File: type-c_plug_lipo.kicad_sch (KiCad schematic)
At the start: 14 parts, among them J1 Conn_Battery, J2 USB_C_Plug_USB2.0, J4 Conn_Pwr, U1 MCP73831

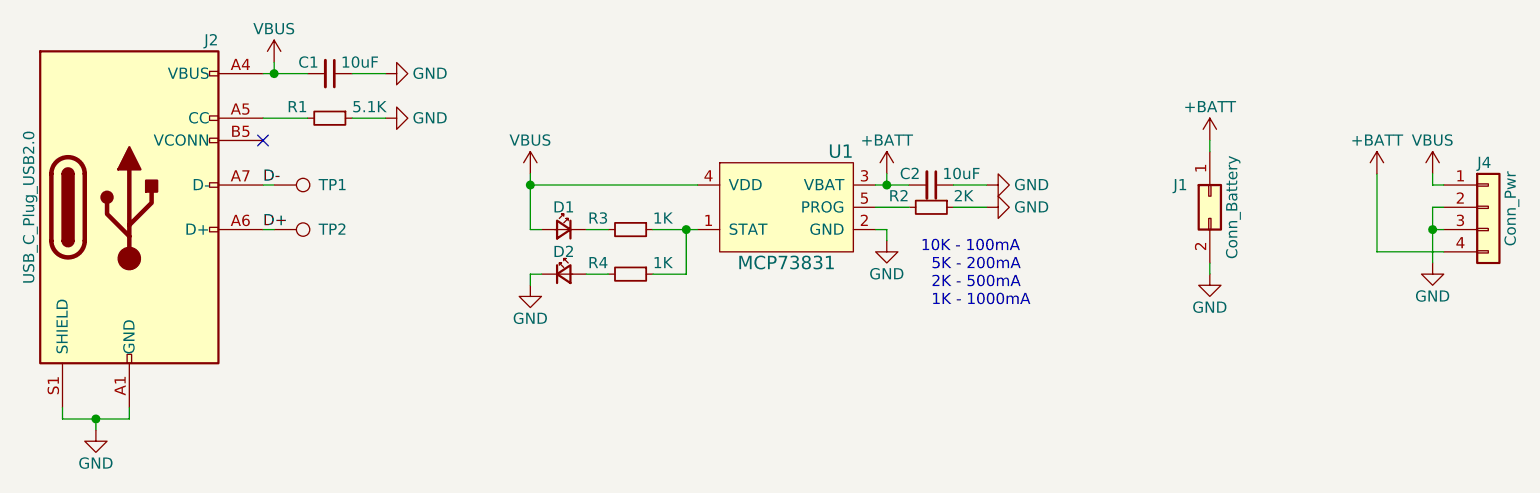
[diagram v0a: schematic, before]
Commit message: Rev 2
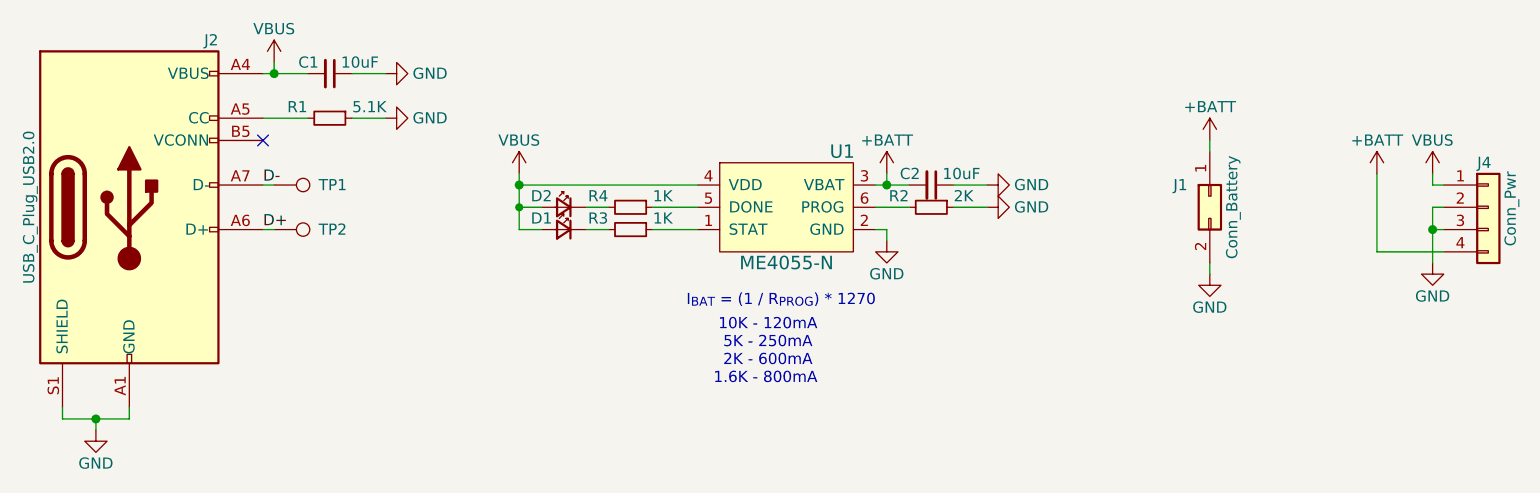
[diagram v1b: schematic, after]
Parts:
- removed U1: MCP73831, Package_TO_SOT_SMD:SOT-23-5, symbol Battery_Management_Extra:MCP73831
- added U1: ME4055-N, Package_TO_SOT_SMD:SOT-23-6, symbol Battery_Management_Extra:ME4055-N
- J1: LCSC C375128 -> C47647
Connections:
- net +BATT: now also U1.3 (VBAT)
- net GND: now also U1.2 (GND); no longer D2.1 (K)
- net VBUS: now also D2.2 (A), U1.4 (VDD)
- net at R4.1: now also U1.5 (DONE); no longer R3.1
- net at R4.2: now also D2.1 (K); no longer D2.2 (A)
- net at R2.2: now also U1.6 (PROG)
- new net: R3.1, U1.1 (STAT)
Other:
- note added: "10K - 120mA 5K - 250mA 2K - 600mA 1.6K - 800mA"
- note added: "I_{BAT} = (1 / R_{PROG}) * 1270"
- note removed: "10K - 100mA"
- note removed: "5K - 200mA 2K - 500mA 1K - 1000mA"
- moved on the sheet: D2, R4
